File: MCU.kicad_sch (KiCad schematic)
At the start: 3 parts, among them U1 STM32U595RITx, U8 ATECC608A-SSHDA

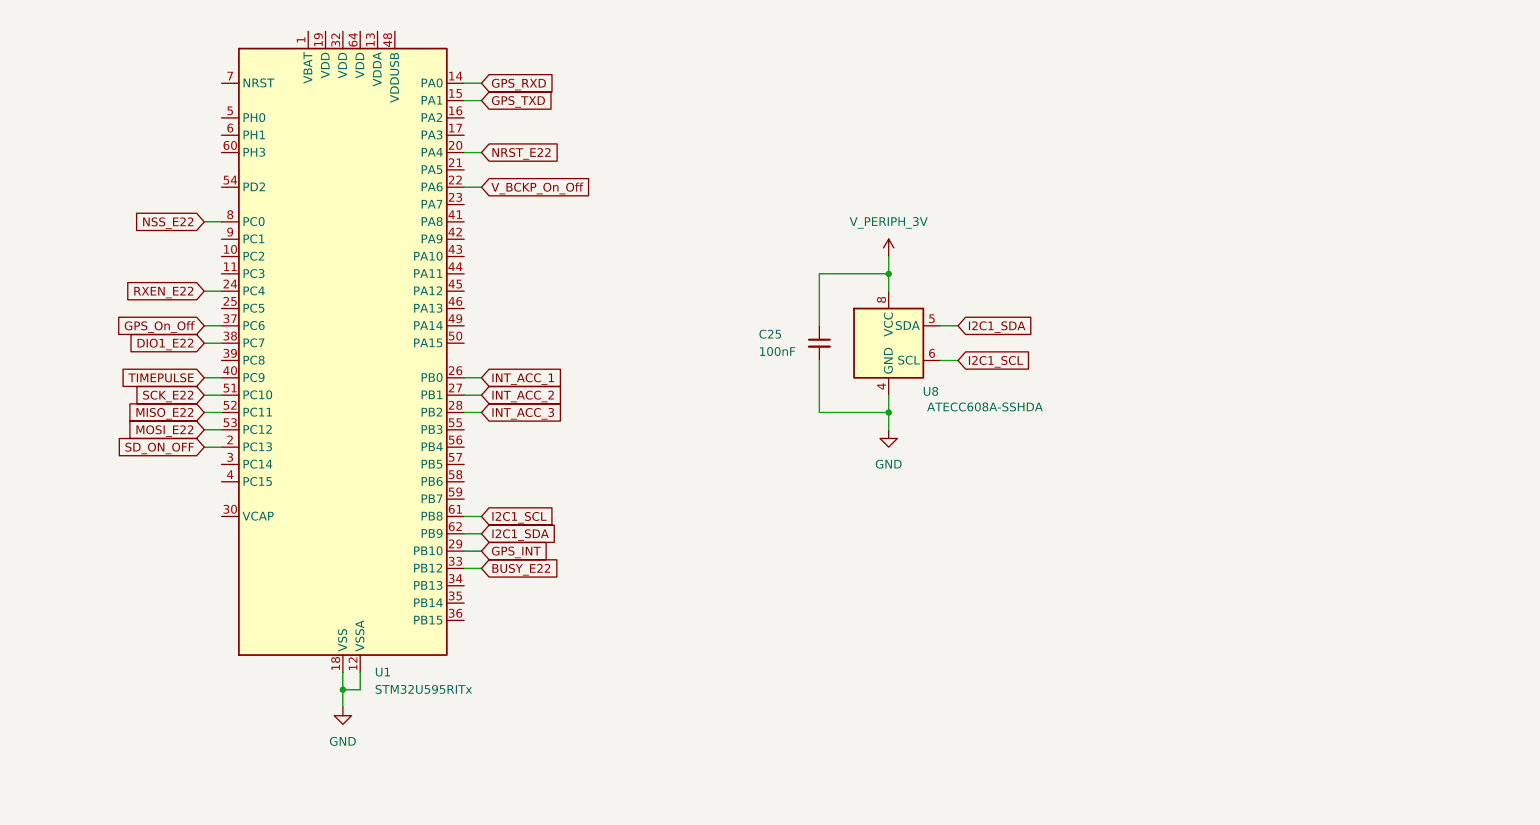
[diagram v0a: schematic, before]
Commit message: Continue filling schematics
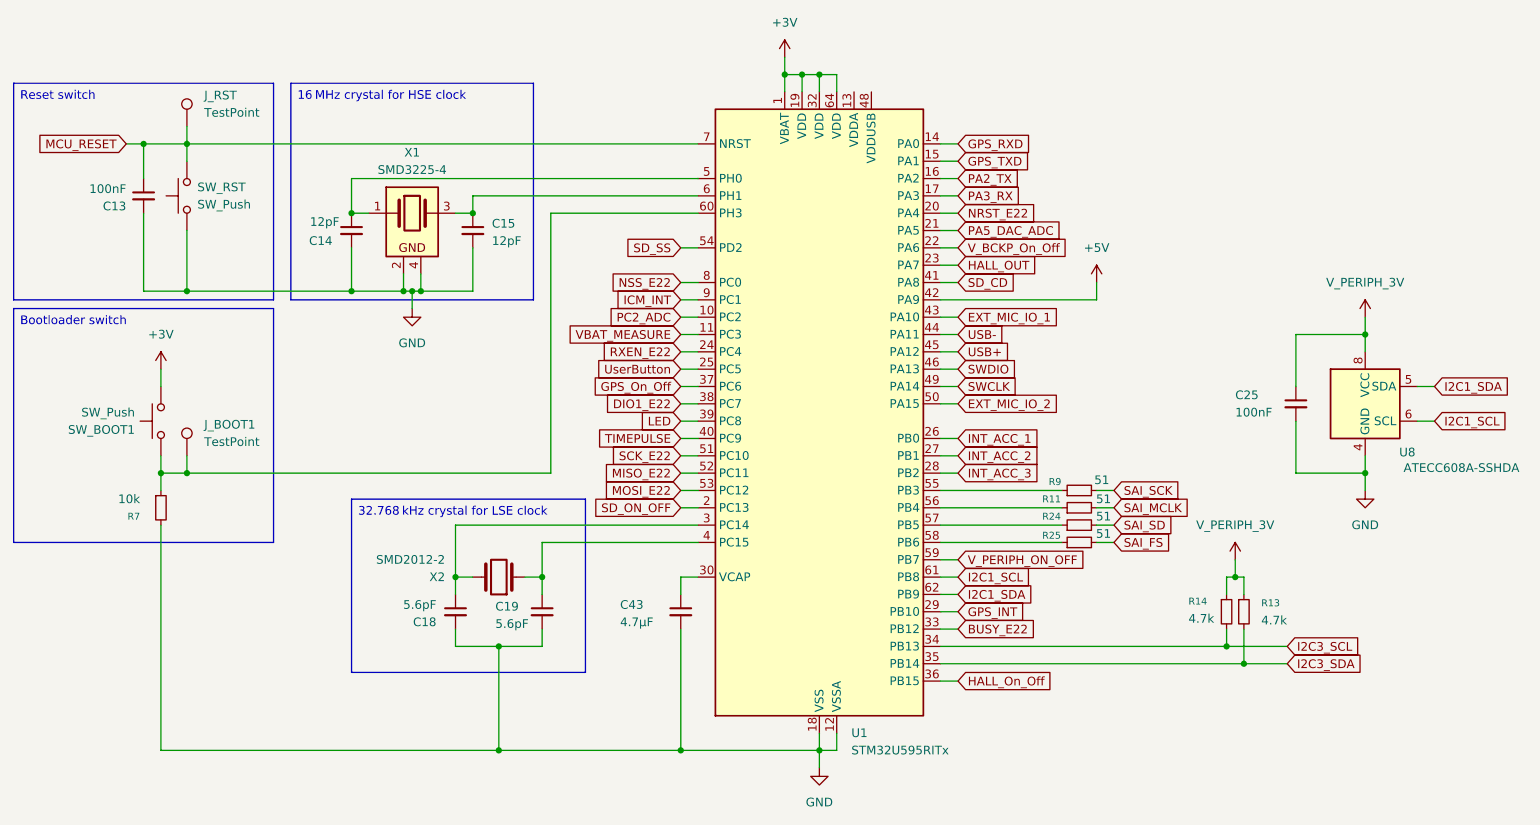
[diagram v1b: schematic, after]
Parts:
- added C13: 100nF, symbol Device:C_Small
- added C14, C15: 12pF, symbol Device:C_Small
- added C18, C19: 5.6pF, symbol Device:C_Small
- added C43: 4.7µF, symbol Device:C_Small
- added J_BOOT1, J_RST: TestPoint, symbol Connector:TestPoint
- added R11, R24, R25, R9: 51, symbol Device:R_Small
- added R13, R14: 4.7k, symbol Device:R_Small
- added R7: 10k, symbol Device:R_Small
- added SW_BOOT1, SW_RST: SW_Push, symbol Switch:SW_Push
- added X1: SMD3225-4, PCM_Crystal_AKL:Crystal_SMD_3225-4Pin_3.2x2.5mm, symbol PCM_Crystal_AKL:SMD3225-4
- added X2: SMD2012-2, PCM_Crystal_AKL:Crystal_SMD_2012-2Pin_2.0x1.2mm, symbol PCM_Crystal_AKL:SMD2012-2
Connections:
- net GND: now also C13.2, C14.2, C15.2, C18.2, C19.2, C43.2, R7.2, SW_RST.1, X1.2, X1.4
- net V_PERIPH_3V: now also R13.1, R14.1
- net +3V: now reaches U1.1 (VBAT)
- net +3V: now also U1.19 (VDD), U1.32 (VDD), U1.64 (VDD), SW_BOOT1.2
- net PC2_ADC: now reaches U1.10 (PC2)
- net VBAT_MEASURE: now reaches U1.11 (PC3)
- net PA2_TX: now reaches U1.16 (PA2)
- net PA3_RX: now reaches U1.17 (PA3)
- net PA5_DAC_ADC: now reaches U1.21 (PA5)
- net HALL_OUT: now reaches U1.23 (PA7)
- net UserButton: now reaches U1.25 (PC5)
- net at U1.3 (PC14): now also C18.1, X2.2
- net at U1.30 (VCAP): now also C43.1
- net I2C3_SCL: now reaches U1.34 (PB13)
- net I2C3_SCL: now also R14.2
- net I2C3_SDA: now reaches U1.35 (PB14)
- net I2C3_SDA: now also R13.2
- net HALL_On_Off: now reaches U1.36 (PB15)
- net LED: now reaches U1.39 (PC8)
- net at U1.4 (PC15): now also C19.1, X2.1
- net SD_CD: now reaches U1.41 (PA8)
- net +5V: now reaches U1.42 (PA9)
- net EXT_MIC_IO_1: now reaches U1.43 (PA10)
- net USB-: now reaches U1.44 (PA11)
- net USB+: now reaches U1.45 (PA12)
- net SWDIO: now reaches U1.46 (PA13)
- net SWCLK: now reaches U1.49 (PA14)
- net at U1.5 (PH0): now also C14.1, X1.1
- net EXT_MIC_IO_2: now reaches U1.50 (PA15)
- net SD_SS: now reaches U1.54 (PD2)
- net at U1.55 (PB3): now also R9.1
- net at U1.56 (PB4): now also R11.1
- net at U1.57 (PB5): now also R24.1
- net at U1.58 (PB6): now also R25.1
- net V_PERIPH_ON_OFF: now reaches U1.59 (PB7)
- net at U1.6 (PH1): now also C15.1, X1.3
- net at U1.60 (PH3): now also J_BOOT1.1, R7.1, SW_BOOT1.1
- net MCU_RESET: now reaches U1.7 (NRST)
- net MCU_RESET: now also C13.1, J_RST.1, SW_RST.2
- net ICM_INT: now reaches U1.9 (PC1)
- new net SAI_FS: R25.2
- new net SAI_MCLK: R11.2
- new net SAI_SCK: R9.2
- new net SAI_SD: R24.2
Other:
- moved on the sheet: C25, U1, U8
